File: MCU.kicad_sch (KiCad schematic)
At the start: 13 parts, among them U1 STM32G474RETx

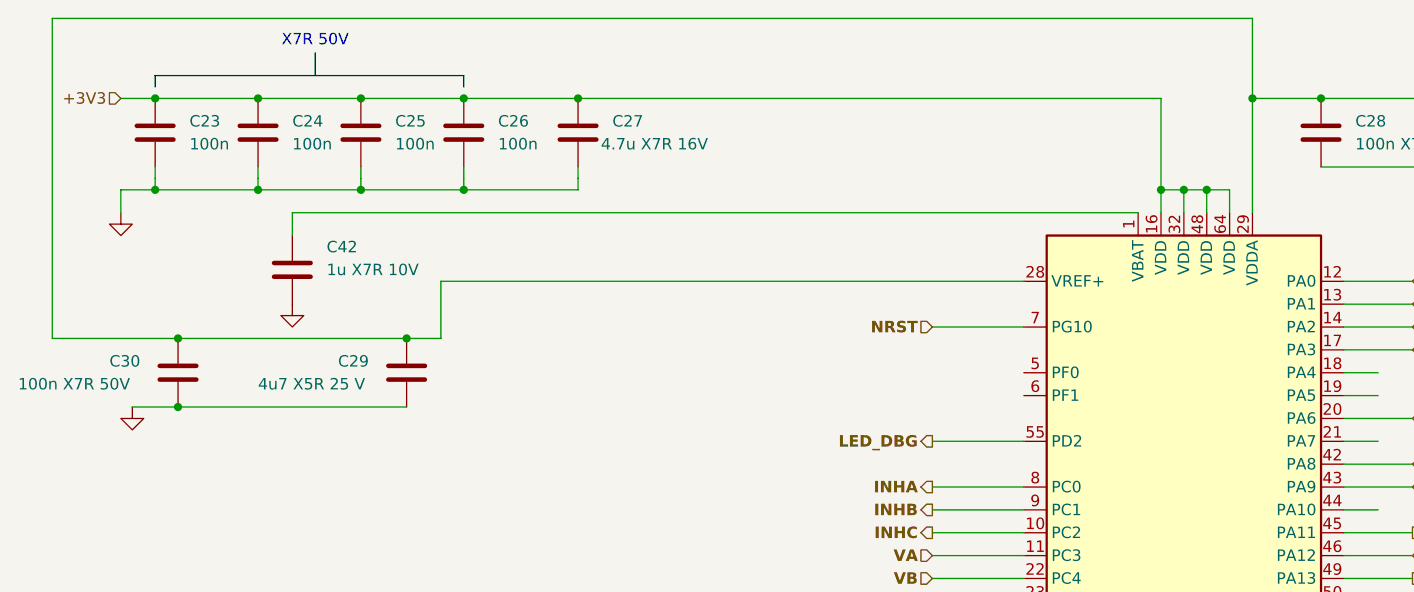
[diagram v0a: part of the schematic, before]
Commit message: verfication inverter
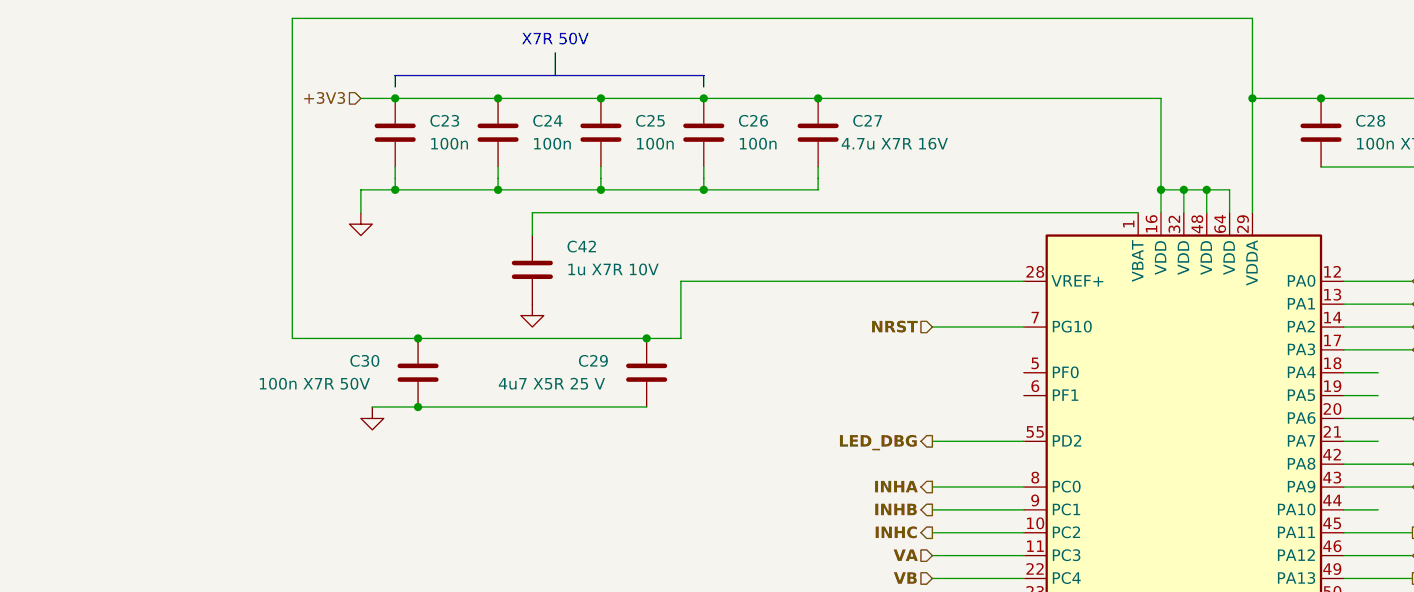
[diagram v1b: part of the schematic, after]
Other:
- moved on the sheet: C23, C24, C25, C26, C27, C29, C30, C42
